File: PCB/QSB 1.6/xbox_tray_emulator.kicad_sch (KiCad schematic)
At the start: 6 parts, among them J1 to Xbox, U1 ATtiny13A-S, U2 AP2127N-3.3

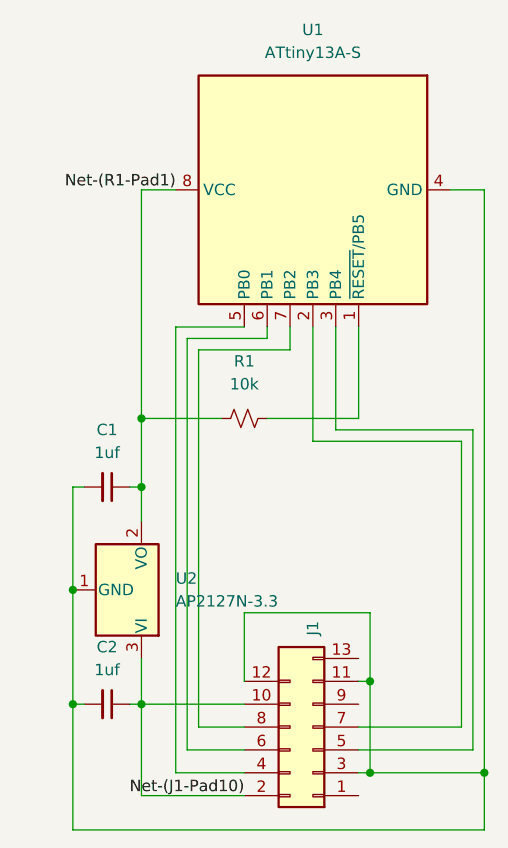
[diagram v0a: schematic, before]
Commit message: add net lables, add firmware, update .gitignore
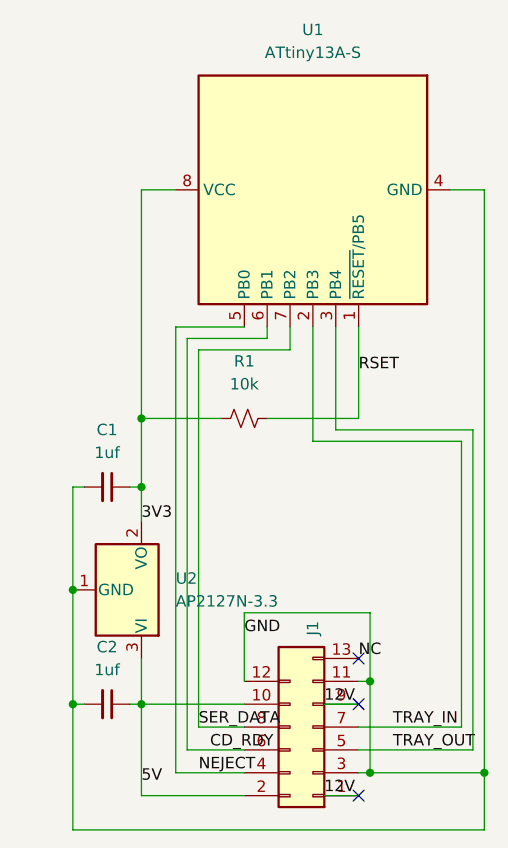
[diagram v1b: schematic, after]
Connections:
- net GND: now reaches C1.2, C2.2, J1.11 (Pin_11), J1.12 (Pin_12), J1.3 (Pin_3), U1.4 (GND), U2.1 (GND)
- net 12V: now reaches J1.1 (Pin_1)
- net 12V: now also J1.9 (Pin_9)
- net NC: now reaches J1.13 (Pin_13)
- net NEJECT: now reaches J1.4 (Pin_4), U1.5 (PB0)
- net TRAY_OUT: now reaches J1.5 (Pin_5), U1.3 (PB4)
- net CD_RDY: now reaches J1.6 (Pin_6), U1.6 (PB1)
- net TRAY_IN: now reaches J1.7 (Pin_7), U1.2 (PB3)
- net SER_DATA: now reaches J1.8 (Pin_8), U1.7 (PB2)
- net RSET: now reaches R1.2, U1.1 (~{RESET}/PB5)
- net Net-(J1-Pad10) renamed 5V
- net Net-(R1-Pad1) renamed 3V3
- no-connect marks 0 -> 3
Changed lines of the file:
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@@
 		(color 0 0 0 0)
 	)
+	(no_connect
+		(at 175.26 142.24)
+	)
+	(no_connect
+		(at 175.26 127)
+	)
+	(no_connect
+		(at 175.26 132.08)
+	)
 	(wire
 		(pts
@@
 	(wire
 		(pts
+			(xy 171.45 142.24) (xy 175.26 142.24)
+		)
+		(stroke
+			(width 0)
+			(type default)
+		)
+	)
+	(wire
+		(pts
 			(xy 167.64 92.71) (xy 157.48 92.71)
 		)
@@
 	(wire
 		(pts
+			(xy 171.45 132.08) (xy 175.26 132.08)
+		)
+		(stroke
+			(width 0)
+			(type default)
+		)
+	)
+	(wire
+		(pts
 			(xy 144.78 132.08) (xy 143.51 132.08)
 		)
@@
 		)
 	)
-	(label "Net-(R1-Pad1)"
-		(at 154.94 74.93 180)
-		(effects
-			(font
-				(size 1.27 1.27)
-			)
-			(justify right bottom)
-		)
-	)
-	(label "Net-(J1-Pad10)"
-		(at 162.56 142.24 180)
-		(effects
-			(font
-				(size 1.27 1.27)
-			)
-			(justify right bottom)
-		)
-	)
+	(label "3V3"
+		(at 151.13 111.76 0)
+		(effects
+			(font
+				(size 1.27 1.27)
+			)
+			(justify left bottom)
+		)
+	)
+	(label "RSET"
+		(at 175.26 95.25 0)
+		(effects
+			(font
+				(size 1.27 1.27)
+			)
+			(justify left bottom)
+		)
+	)
+	(label "NC"
+		(at 175.26 127 0)
+		(effects
+			(font
+				(size 1.27 1.27)
+			)
+			(justify left bottom)
+		)
+	)
+	(label "12V"
+		(at 171.45 132.08 0)
+		(effects
+			(font
+				(size 1.27 1.27)
+			)
+			(justify left bottom)
+		)
+	)
+	(label "NEJECT"
+		(at 157.48 139.7 0)
+		(effects
+			(font
+				(size 1.27 1.27)
+			)
+			(justify left bottom)
+		)
+	)
+	(label "5V"
+		(at 151.13 140.97 0)
+		(effects
+			(font
+				(size 1.27 1.27)
+			)
+			(justify left bottom)
+		)
+	)
+	(label "TRAY_OUT"
+		(at 179.07 137.16 0)
+		(effects
+			(font
+				(size 1.27 1.27)
+			)
+			(justify left bottom)
+		)
+	)
+	(label "GND"
+		(at 162.56 124.46 0)
+		(effects
+			(font
+				(size 1.27 1.27)
+			)
+			(justify left bottom)
+		)
+	)
+	(label "SER_DATA"
+		(at 157.48 134.62 0)
+		(effects
+			(font
+				(size 1.27 1.27)
+			)
+			(justify left bottom)
+		)
+	)
+	(label "12V"
+		(at 171.45 142.24 0)
+		(effects
+			(font
+				(size 1.27 1.27)
+			)
+			(justify left bottom)
+		)
+	)
+	(label "TRAY_IN"
+		(at 179.07 134.62 0)
+		(effects
+			(font
+				(size 1.27 1.27)
+			)
+			(justify left bottom)
+		)
+	)
+	(label "CD_RDY"
+		(at 158.75 137.16 0)
+		(effects
+			(font
+				(size 1.27 1.27)
+			)
+			(justify left bottom)
+		)
+	)
